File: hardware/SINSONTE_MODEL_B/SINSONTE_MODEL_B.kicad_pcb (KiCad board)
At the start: 2 copper layers, 90 x 41 mm, 42 parts, among them J1 BAT, J10 Conn_01x02_Male, J11 Conn_01x02_Male, J12 Conn_01x02_Male, J13 Conn_01x02_Male, J14 Conn_01x02_Male, J15 Conn_01x02_Male, J16 Conn_01x02_Male, J17 Conn_01x02_Male, J18 Conn_01x02_Male, J2 CLOCK, J3 PROG, J4 LIGHT_SENSOR, J5 Conn_01x20_Male, J6 Conn_01x20_Male, J7 Conn_01x05_Male, J8 Conn_01x05_Male, J9 Conn_01x02_Male, Q1 2N7000, Q2 PN2222A, SW1 SW_Push, U1 Pico

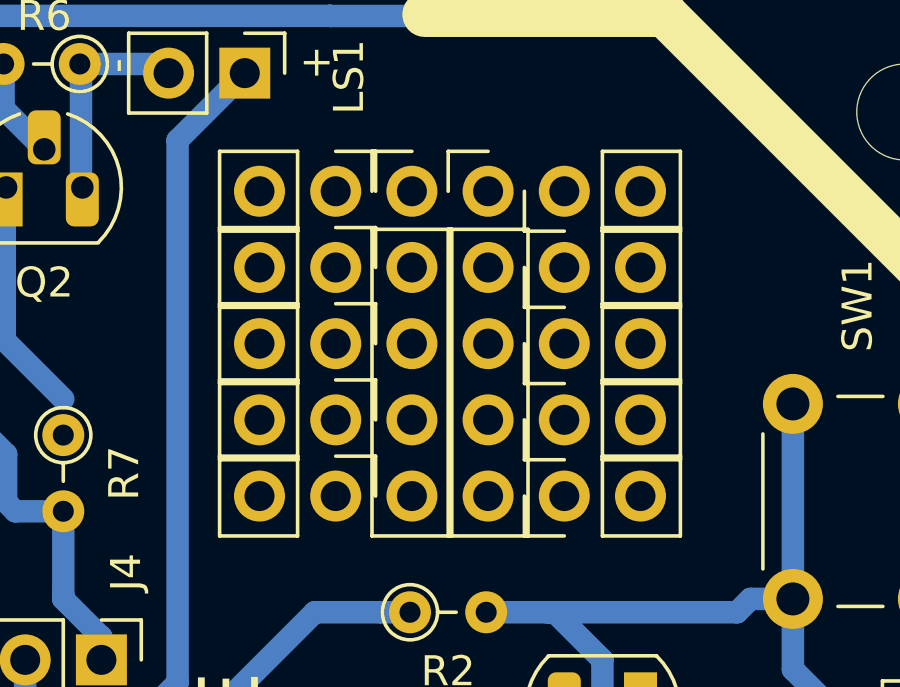
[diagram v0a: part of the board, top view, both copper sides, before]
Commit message: single gerber proto fix
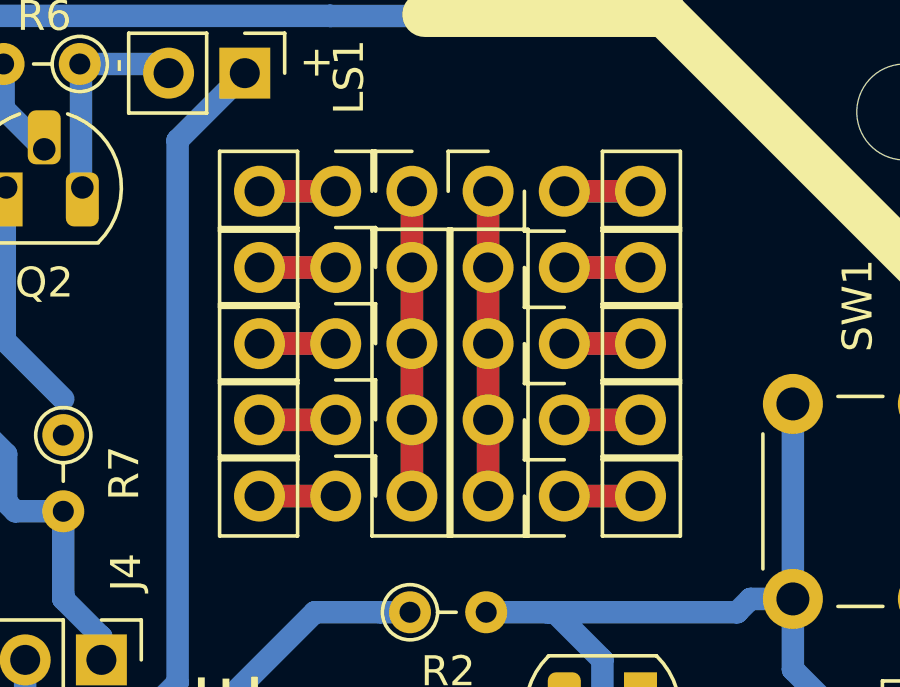
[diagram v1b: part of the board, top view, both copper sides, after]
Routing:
- net Net-(J8-Pad1): track 0.00 -> 20.3 mm
- net Net-(J7-Pad1): track 0.00 -> 20.3 mm
- net Net-(J9-Pad1): track 0.00 -> 5.08 mm
- net Net-(J18-Pad1): track 0.00 -> 5.08 mm
- net Net-(J17-Pad1): track 0.00 -> 5.08 mm
- net Net-(J16-Pad1): track 0.00 -> 5.08 mm
- net Net-(J15-Pad1): track 0.00 -> 5.08 mm
- net Net-(J14-Pad1): track 0.00 -> 5.08 mm
- net Net-(J13-Pad1): track 0.00 -> 5.08 mm
- net Net-(J12-Pad1): track 0.00 -> 5.08 mm
- net Net-(J11-Pad1): track 0.00 -> 5.08 mm
- net Net-(J10-Pad1): track 0.00 -> 5.08 mm
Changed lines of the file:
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@@
     (thickness 1.6)
     (drawings 21)
-    (tracks 225)
+    (tracks 261)
     (zones 0)
     (modules 42)
@@
   (segment (start 53.34 74.93) (end 52.07 76.2) (width 0.75) (layer B.Cu) (net 41))
   (segment (start 53.87 60.11) (end 53.87 57.57) (width 0.75) (layer B.Cu) (net 42))
+  (segment (start 119.5705 56.642) (end 119.5705 59.182) (width 0.75) (layer F.Cu) (net 43))
+  (segment (start 119.5705 59.182) (end 119.5705 61.722) (width 0.75) (layer F.Cu) (net 43))
+  (segment (start 119.5705 61.722) (end 119.5705 64.262) (width 0.75) (layer F.Cu) (net 43))
+  (segment (start 119.5705 66.802) (end 119.5705 64.262) (width 0.75) (layer F.Cu) (net 43))
+  (segment (start 119.5705 56.642) (end 119.5705 59.182) (width 0.75) (layer B.Cu) (net 43))
+  (segment (start 119.5705 59.182) (end 119.5705 61.722) (width 0.75) (layer B.Cu) (net 43))
+  (segment (start 119.5705 61.722) (end 119.5705 64.262) (width 0.75) (layer B.Cu) (net 43))
+  (segment (start 119.5705 64.262) (end 119.5705 66.802) (width 0.75) (layer B.Cu) (net 43))
+  (segment (start 122.1105 56.642) (end 122.1105 59.182) (width 0.75) (layer F.Cu) (net 44))
+  (segment (start 122.1105 59.182) (end 122.1105 61.722) (width 0.75) (layer F.Cu) (net 44))
+  (segment (start 122.1105 61.722) (end 122.1105 64.262) (width 0.75) (layer F.Cu) (net 44))
+  (segment (start 122.1105 64.262) (end 122.1105 66.802) (width 0.75) (layer F.Cu) (net 44))
+  (segment (start 122.1105 56.642) (end 122.1105 59.182) (width 0.75) (layer B.Cu) (net 44))
+  (segment (start 122.1105 59.182) (end 122.1105 61.722) (width 0.75) (layer B.Cu) (net 44))
+  (segment (start 122.1105 61.722) (end 122.1105 64.262) (width 0.75) (layer B.Cu) (net 44))
+  (segment (start 122.1105 64.262) (end 122.1105 66.802) (width 0.75) (layer B.Cu) (net 44))
+  (segment (start 114.4905 66.802) (end 117.0305 66.802) (width 0.75) (layer F.Cu) (net 45))
+  (segment (start 114.4905 66.802) (end 117.0305 66.802) (width 0.75) (layer B.Cu) (net 45))
+  (segment (start 114.4905 64.262) (end 117.0305 64.262) (width 0.75) (layer F.Cu) (net 46))
+  (segment (start 114.4905 64.262) (end 117.0305 64.262) (width 0.75) (layer B.Cu) (net 46))
+  (segment (start 114.4905 61.722) (end 117.0305 61.722) (width 0.75) (layer F.Cu) (net 47))
+  (segment (start 114.4905 61.722) (end 117.0305 61.722) (width 0.75) (layer B.Cu) (net 47))
+  (segment (start 114.4905 59.182) (end 117.0305 59.182) (width 0.75) (layer F.Cu) (net 48))
+  (segment (start 114.4905 59.182) (end 117.0305 59.182) (width 0.75) (layer B.Cu) (net 48))
+  (segment (start 114.4905 56.642) (end 117.0305 56.642) (width 0.75) (layer F.Cu) (net 49))
+  (segment (start 114.4905 56.642) (end 117.0305 56.642) (width 0.75) (layer B.Cu) (net 49))
+  (segment (start 124.6505 66.802) (end 127.1905 66.802) (width 0.75) (layer F.Cu) (net 50))
+  (segment (start 124.6505 66.802) (end 127.1905 66.802) (width 0.75) (layer B.Cu) (net 50))
+  (segment (start 124.6505 64.262) (end 127.1905 64.262) (width 0.75) (layer F.Cu) (net 51))
+  (segment (start 124.6505 64.262) (end 127.1905 64.262) (width 0.75) (layer B.Cu) (net 51))
+  (segment (start 124.6505 61.722) (end 127.1905 61.722) (width 0.75) (layer F.Cu) (net 52))
+  (segment (start 124.6505 61.722) (end 127.1905 61.722) (width 0.75) (layer B.Cu) (net 52))
+  (segment (start 124.6505 59.182) (end 127.1905 59.182) (width 0.75) (layer F.Cu) (net 53))
+  (segment (start 124.6505 59.182) (end 127.1905 59.182) (width 0.75) (layer B.Cu) (net 53))
+  (segment (start 124.6505 56.642) (end 127.1905 56.642) (width 0.75) (layer F.Cu) (net 54))
+  (segment (start 124.6505 56.642) (end 127.1905 56.642) (width 0.75) (layer B.Cu) (net 54))
   (zone (net 4) (net_name "Net-(BT1-Pad2)") (layer B.Cu) (hatch edge 0.508)
     (connect_pads (clearance 0.508))
